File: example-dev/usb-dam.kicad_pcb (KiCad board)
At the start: 2 copper layers, 39 x 25 mm, 42 parts, among them J1 USB_C_Receptacle, J2 Conn_01x08_Pin, U1 MCP6002-xMC, U2 SiP32431DR3, U3 TMUX1574RSVR, U4 74LVC1G08

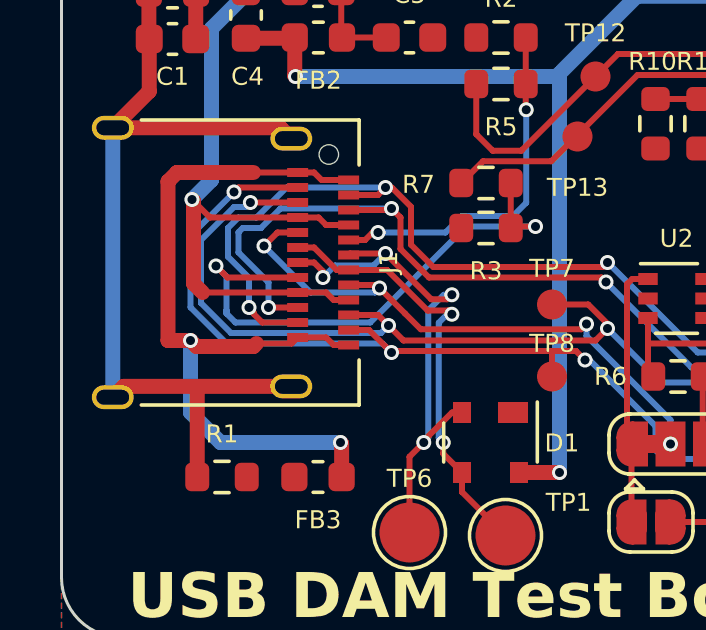
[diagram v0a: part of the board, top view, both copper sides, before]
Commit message: pcb render
active layers
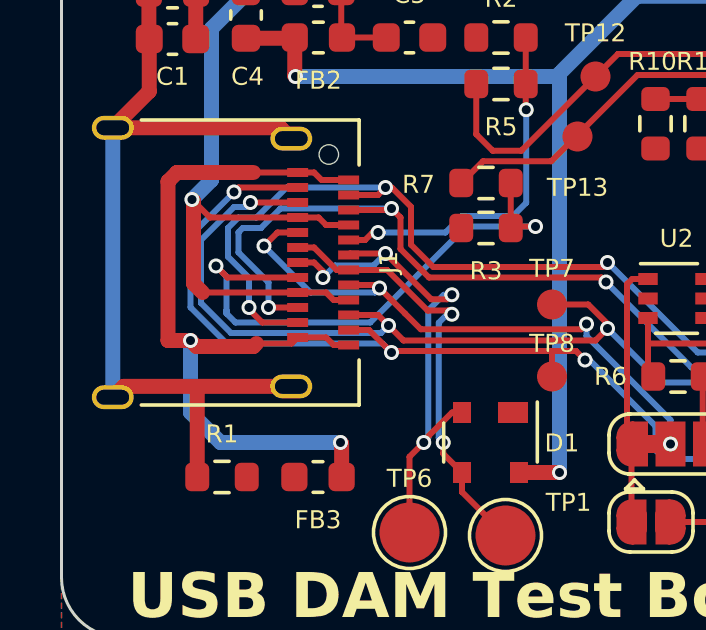
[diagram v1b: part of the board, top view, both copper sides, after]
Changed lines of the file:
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@@
   (segment (start 117.007107 88) (end 117.65 88.642893) (width 0.2) (layer "F.Cu") (net 9))
   (segment (start 124.05 90.65) (end 124.2 90.5) (width 0.2) (layer "F.Cu") (net 9))
-  (segment (start 112.4 92.149503) (end 112.4 92.207107) (width 0.2) (layer "F.Cu") (net 9))
   (segment (start 129.65 92.6) (end 129.65 93.493393) (width 0.2) (layer "F.Cu") (net 9))
   (segment (start 116.55 88.25) (end 115.57 88.25) (width 0.2) (layer "F.Cu") (net 9))
-  (segment (start 112.4 92.207107) (end 112.692893 92.5) (width 0.2) (layer "F.Cu") (net 9))
+  (segment (start 112.250497 92) (end 112.250497 92.057604) (width 0.2) (layer "F.Cu") (net 9))
+  (segment (start 112.692893 92.5) (end 113.87 92.5) (width 0.2) (layer "F.Cu") (net 9))
   (segment (start 130.206607 94.05) (end 130.85 94.05) (width 0.2) (layer "F.Cu") (net 9))
+  (segment (start 112.250497 92.057604) (end 112.692893 92.5) (width 0.2) (layer "F.Cu") (net 9))
   (segment (start 129.65 93.493393) (end 129.656607 93.5) (width 0.2) (layer "F.Cu") (net 9))
   (segment (start 129.656607 93.5) (end 130.206607 94.05) (width 0.2) (layer "F.Cu") (net 9))
-  (segment (start 112.250497 92) (end 112.4 92.149503) (width 0.2) (layer "F.Cu") (net 9))
   (segment (start 117.65 88.642893) (end 117.65 89.905026) (width 0.2) (layer "F.Cu") (net 9))
   (segment (start 116.8 88) (end 117.007107 88) (width 0.2) (layer "F.Cu") (net 9))
-  (segment (start 112.692893 92.5) (end 113.87 92.5) (width 0.2) (layer "F.Cu") (net 9))
   (via (at 112.250497 92) (size 0.5) (drill 0.3) (layers "F.Cu" "B.Cu") (net 9))
   (via (at 124.2 90.5) (size 0.5) (drill 0.3) (layers "F.Cu" "B.Cu") (net 9))
